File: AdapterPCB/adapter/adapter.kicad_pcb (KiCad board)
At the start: 2 copper layers, 60.5 x 44.5 mm, 21 parts, among them J2 VGA, U1 SN74LVC245APW, U2 SN74LVC245APW

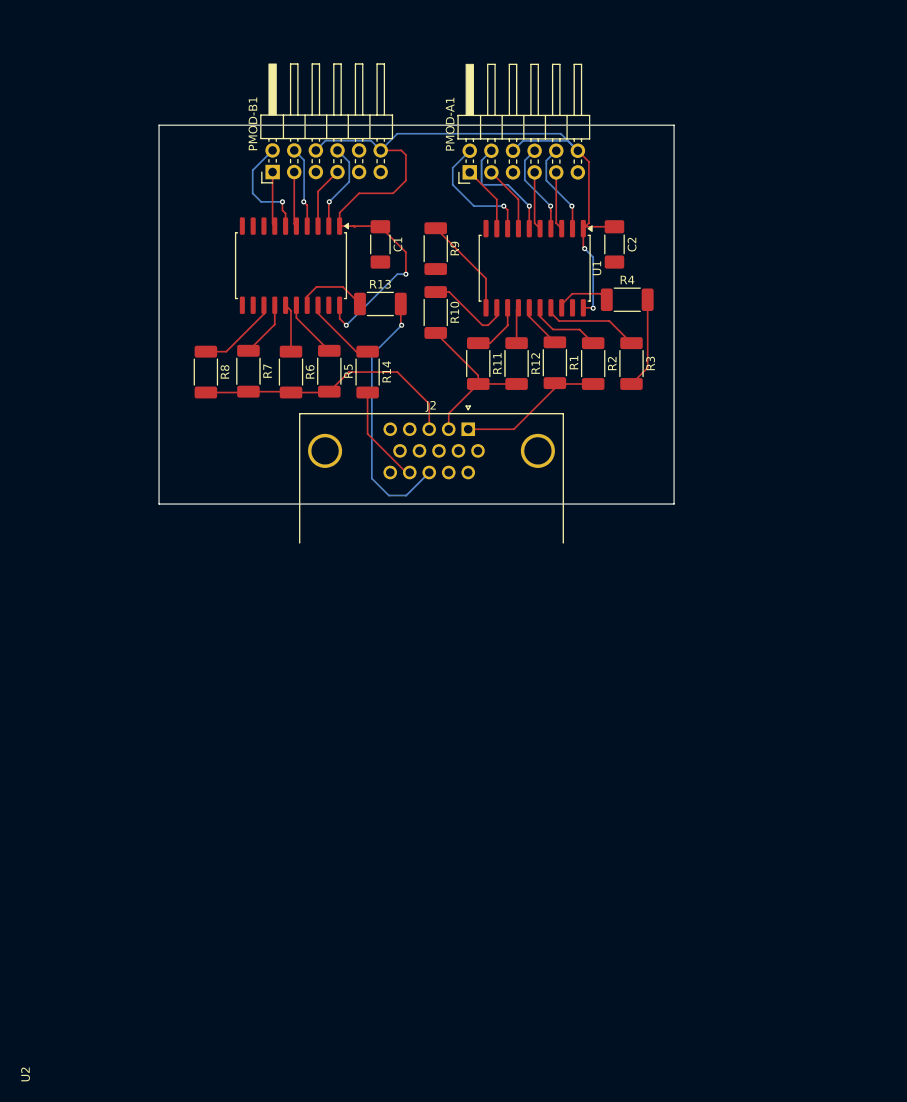
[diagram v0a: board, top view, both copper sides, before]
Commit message: ye
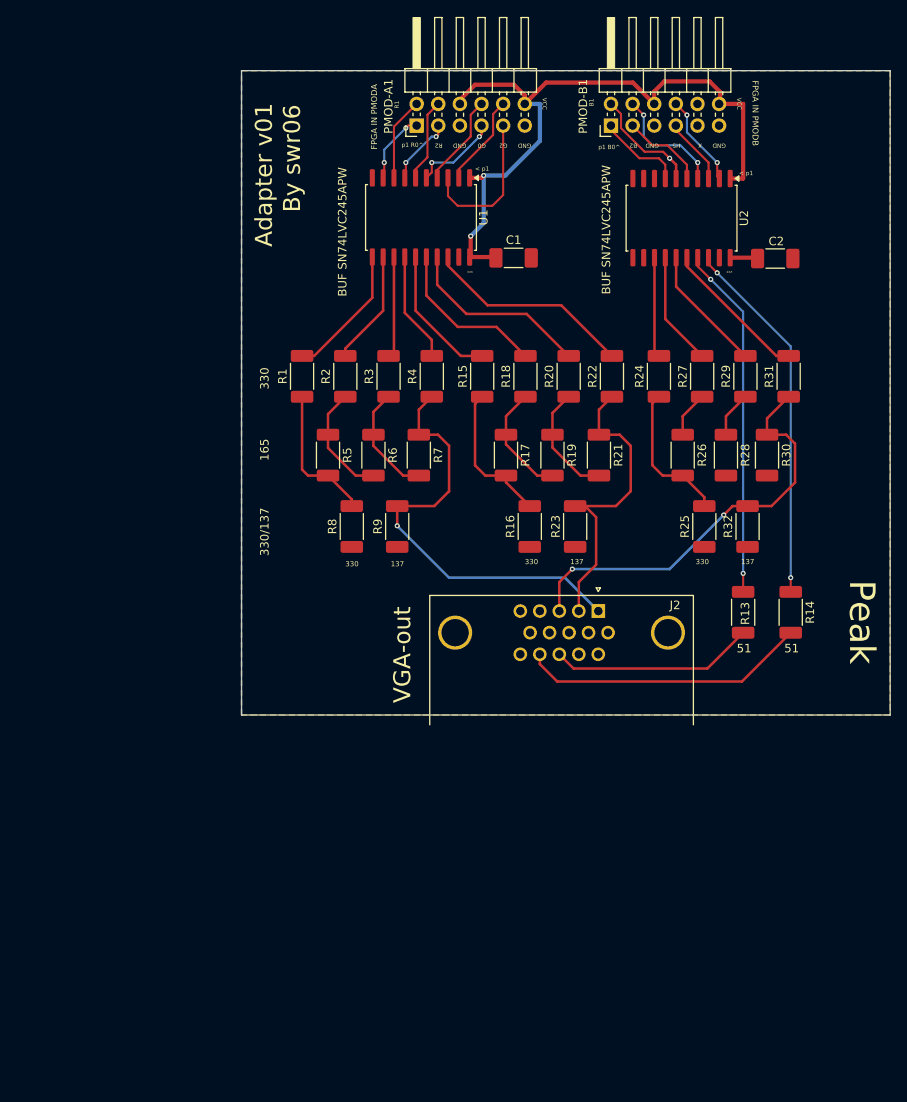
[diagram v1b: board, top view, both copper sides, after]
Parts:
- removed R10: 1k, Resistor_SMD:R_2010_5025Metric_Pad1.40x2.65mm_HandSolder
- removed R11: 2k, Resistor_SMD:R_2010_5025Metric_Pad1.40x2.65mm_HandSolder
- removed R12: 4.02k, Resistor_SMD:R_2010_5025Metric_Pad1.40x2.65mm_HandSolder
- added R15: 330, Resistor_SMD:R_2010_5025Metric_Pad1.40x2.65mm_HandSolder, F.Cu at (135.5, 81.5)
- added R16: 330, Resistor_SMD:R_2010_5025Metric_Pad1.40x2.65mm_HandSolder, F.Cu at (141.0, 99.1)
- added R17: 165, Resistor_SMD:R_2010_5025Metric_Pad1.40x2.65mm_HandSolder, F.Cu at (138.3, 90.8)
- added R18: 330, Resistor_SMD:R_2010_5025Metric_Pad1.40x2.65mm_HandSolder, F.Cu at (140.5, 81.5)
- added R19: 165, Resistor_SMD:R_2010_5025Metric_Pad1.40x2.65mm_HandSolder, F.Cu at (143.7, 90.8)
- added R20: 330, Resistor_SMD:R_2010_5025Metric_Pad1.40x2.65mm_HandSolder, F.Cu at (145.6, 81.5)
- added R21: 165, Resistor_SMD:R_2010_5025Metric_Pad1.40x2.65mm_HandSolder, F.Cu at (149.2, 90.8)
- added R22: 330, Resistor_SMD:R_2010_5025Metric_Pad1.40x2.65mm_HandSolder, F.Cu at (150.7, 81.5)
- added R23: 137, Resistor_SMD:R_2010_5025Metric_Pad1.40x2.65mm_HandSolder, F.Cu at (146.4, 99.1)
- added R24: 330, Resistor_SMD:R_2010_5025Metric_Pad1.40x2.65mm_HandSolder, F.Cu at (156.2, 81.5)
- added R25: 330, Resistor_SMD:R_2010_5025Metric_Pad1.40x2.65mm_HandSolder, F.Cu at (161.6, 99.1)
- added R26: 165, Resistor_SMD:R_2010_5025Metric_Pad1.40x2.65mm_HandSolder, F.Cu at (159.0, 90.8)
- added R27: 330, Resistor_SMD:R_2010_5025Metric_Pad1.40x2.65mm_HandSolder, F.Cu at (161.3, 81.5)
- added R28: 165, Resistor_SMD:R_2010_5025Metric_Pad1.40x2.65mm_HandSolder, F.Cu at (164.1, 90.8)
- added R29: 330, Resistor_SMD:R_2010_5025Metric_Pad1.40x2.65mm_HandSolder, F.Cu at (166.4, 81.5)
- added R30: 165, Resistor_SMD:R_2010_5025Metric_Pad1.40x2.65mm_HandSolder, F.Cu at (168.9, 90.8)
- added R31: 330, Resistor_SMD:R_2010_5025Metric_Pad1.40x2.65mm_HandSolder, F.Cu at (171.5, 81.5)
- added R32: 137, Resistor_SMD:R_2010_5025Metric_Pad1.40x2.65mm_HandSolder, F.Cu at (166.6, 99.1)
- R1: value 499 -> 330
- R2: value 1k -> 330
- R3: value 2k -> 330
- R4, R8: value 4.02k -> 330
- R5: value 499 -> 165
- R6: value 1k -> 165
- R7: value 2k -> 165
- R9: value 499 -> 137
- moved R14 57.2 mm to (171.7, 109.2)
- moved R13 55.9 mm to (166.1, 109.2), turned to -90 degrees
- moved U2 46.2 mm to (158.9, 62.9)
- moved PMOD-B1 40.1 mm to (150.6, 52.0)
- moved R9 33.0 mm to (125.5, 99.1), turned to 90 degrees
- moved R1 29.7 mm to (114.3, 81.5), turned to 90 degrees
- moved R2 29.2 mm to (119.4, 81.5), turned to 90 degrees
- moved R3 28.6 mm to (124.5, 81.5), turned to 90 degrees
- moved J2 26.3 mm to (149.1, 109.1)
- moved R8 25.0 mm to (120.1, 99.1), turned to 90 degrees
- moved R4 24.7 mm to (129.5, 81.5), turned to 90 degrees
- moved R7 22.3 mm to (128.0, 90.8)
- moved C2 19.0 mm to (169.9, 67.7), turned to 0 degrees
- moved C1 15.7 mm to (139.1, 67.6), turned to 0 degrees
- moved U1 14.6 mm to (128.3, 62.8)
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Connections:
- R1 pad 1: Rb3 -> Net-(R1-Pad1)
- R1 pad 2: AnalogR -> Rb0
- R2 pad 1: Rb2 -> Net-(R2-Pad1)
- R2 pad 2: AnalogR -> Rb1
- R3 pad 1: Rb1 -> Net-(R3-Pad1)
- R3 pad 2: AnalogR -> Rb2
- R4 pad 1: Rb0 -> AnalogR
- R4 pad 2: AnalogR -> Rb3
- R5 pad 1: Bb3 -> Net-(R2-Pad1)
- R5 pad 2: AnalogB -> Net-(R1-Pad1)
- R6 pad 1: Bb2 -> Net-(R3-Pad1)
- R6 pad 2: AnalogB -> Net-(R2-Pad1)
- R7 pad 1: Bb1 -> AnalogR
- R7 pad 2: AnalogB -> Net-(R3-Pad1)
- R8 pad 1: Bb0 -> GND
- R8 pad 2: AnalogB -> Net-(R1-Pad1)
- R9 pad 1: Gb3 -> GND
- R9 pad 2: AnalogG -> AnalogR
- U1 pad 11: Gb3 -> Rb0
- U1 pad 12: Gb2 -> Rb1
- U1 pad 13: Gb1 -> Rb2
- U1 pad 14: Gb0 -> Rb3
- U1 pad 15: Rb3 -> Gb0
- U1 pad 16: Rb2 -> Gb1
- U1 pad 17: Rb1 -> Gb2
- U1 pad 18: Rb0 -> Gb3
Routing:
- net VSyncb: track 8.64 -> 43.3 mm, vias 0 -> 2
- net HSyncb: track 8.53 -> 41.5 mm, vias 0 -> 2
- net AnalogR: track 28.1 -> 51.4 mm, vias 0 -> 1
- net VCC33: track 108.3 -> 85.2 mm, vias 4 -> 2
- net Net-(J2-Pad14): track 11.7 -> 33.8 mm
- net AnalogB: track 31.8 -> 49.7 mm, vias 0 -> 2
- net AnalogG: track 19.3 -> 36.8 mm
- net Net-(R15-Pad1): track 0.00 -> 17.3 mm
- net Net-(R24-Pad1): track 0.00 -> 17.1 mm
- net Net-(R1-Pad1): track 0.00 -> 16.6 mm
- net Net-(R19-Pad1): track 0.00 -> 13.6 mm
- net Net-(R2-Pad1): track 0.00 -> 13.5 mm
- net Net-(R17-Pad1): track 0.00 -> 13.5 mm
- net Net-(R3-Pad1): track 0.00 -> 13.4 mm
- net Gb3: track 11.8 -> 24.7 mm
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- added copper zone on B.Cu, net GND
- added copper zone on F.Cu, net GND
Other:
- board size 60.5 x 44.5 mm -> 76.2 x 75.7 mm
- board text added: "137"
- board text added: "165"
- board text added: "330"
- board text added: "330/137"
- board text added: "51"
- board text added: "< p1"
- board text added: "Adapter v01"
- board text added: "B1"
- board text added: "B2"
- board text added: "BUF SN74LVC245APW"
- board text added: "By swr06"
- board text added: "FPGA IN PMODA"
- board text added: "FPGA IN PMODB"
- board text added: "G0"
- board text added: "G2"
- board text added: "GND"
- board text added: "HS"
- board text added: "Peak"
- board text added: "R1"
- board text added: "R2"
- board text added: "VCC"
- board text added: "VGA-out"
- board text added: "X"
- board text added: "p1 B0^"
- board text added: "p1 R0^"
- board text added: "vcc"
